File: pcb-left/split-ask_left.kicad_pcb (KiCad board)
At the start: 2 copper layers, 165.4 x 98.7 mm, 59 parts, among them J1 MJ-4PP-9, SW1 SW_PUSH, SW10 SW_PUSH, SW11 SW_PUSH, SW12 SW_PUSH, SW13 SW_PUSH, SW14 SW_PUSH, SW15 SW_PUSH, SW16 SW_PUSH, SW17 SW_PUSH, SW18 SW_PUSH, SW19 SW_PUSH, SW2 SW_PUSH, SW20 SW_PUSH, SW21 SW_PUSH, SW22 SW_PUSH, SW23 SW_PUSH, SW24 SW_PUSH, SW25 SW_PUSH, SW26 SW_PUSH, SW27 SW_PUSH, SW28 SW_PUSH, SW3 SW_PUSH, SW4 SW_PUSH, SW5 SW_PUSH, SW6 SW_PUSH, SW7 SW_PUSH, SW8 SW_PUSH, SW9 SW_PUSH, U1 ProMicro

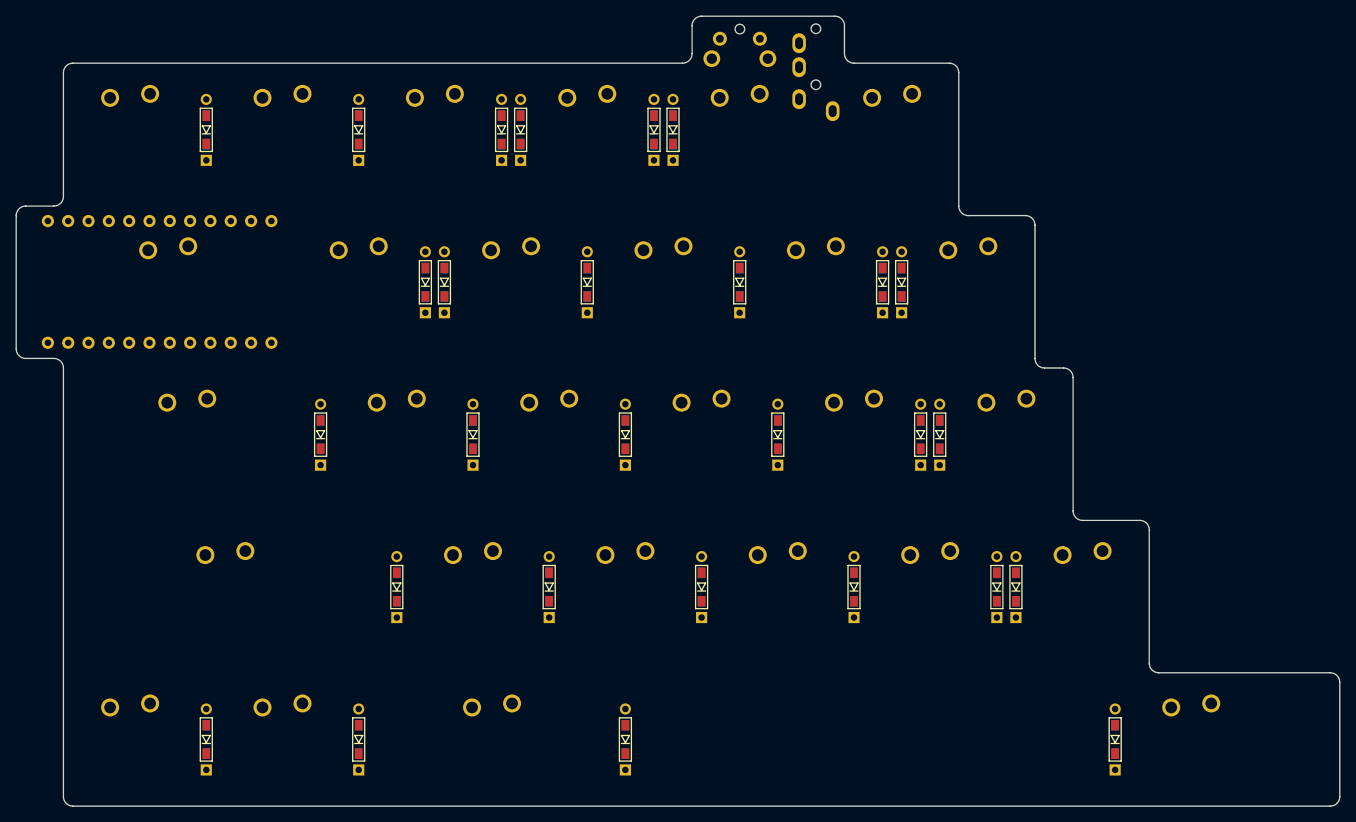
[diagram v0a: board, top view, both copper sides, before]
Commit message: routing
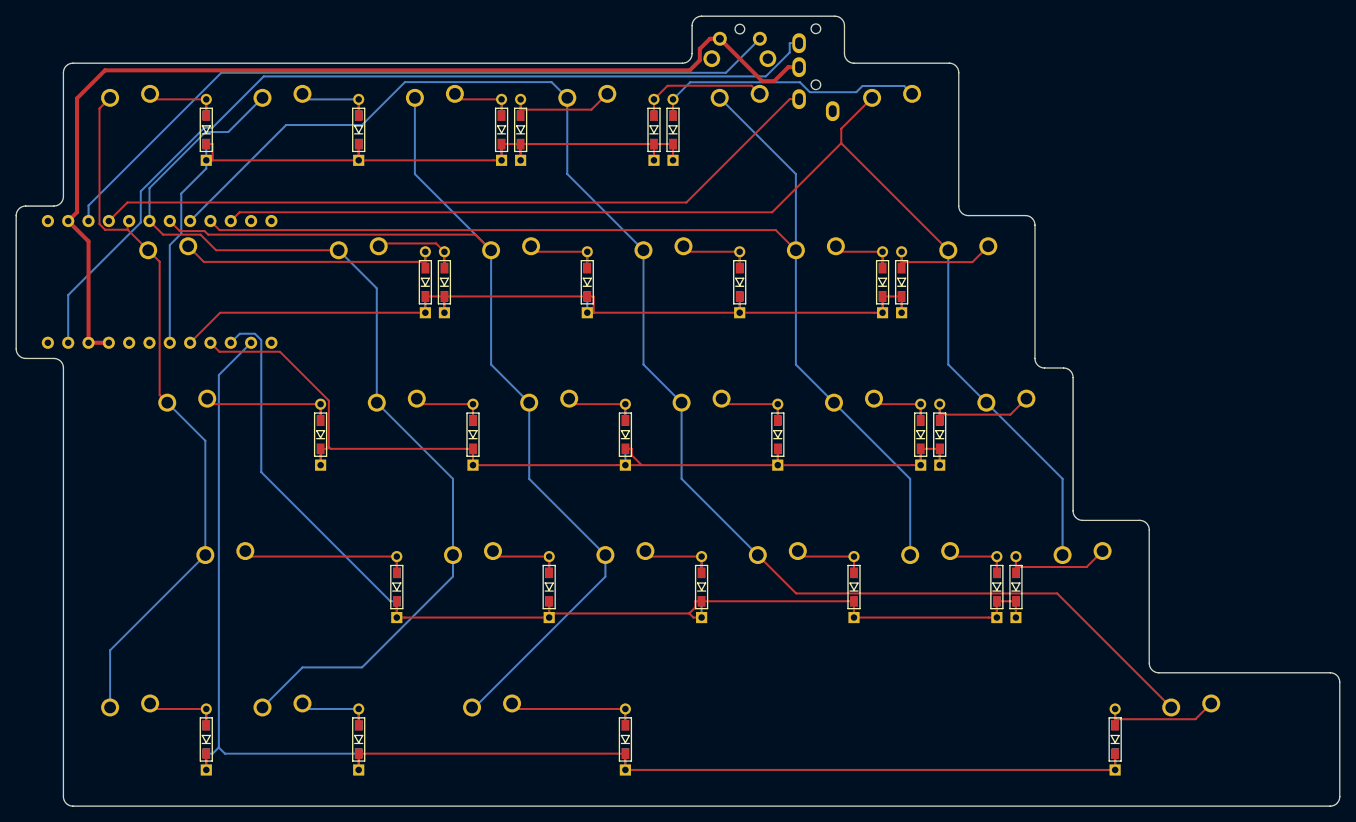
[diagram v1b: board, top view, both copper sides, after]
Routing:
- net row4: track 0.00 -> 183.2 mm
- net col3: track 0.00 -> 181.7 mm
- net col5: track 0.00 -> 150.5 mm
- net row3: track 0.00 -> 147.6 mm
- net col4: track 0.00 -> 141.7 mm
- net col2: track 0.00 -> 134.8 mm
- net GND: track 0.00 -> 131.7 mm
- net row2: track 0.00 -> 126.9 mm
- net col1: track 0.00 -> 125.4 mm
- net row1: track 0.00 -> 115.7 mm
- net data: track 0.00 -> 113.3 mm
- net row0: track 0.00 -> 108.3 mm
- net reset: track 0.00 -> 94.5 mm
- net VCC: track 0.00 -> 92.6 mm
- net col0: track 0.00 -> 90.0 mm
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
